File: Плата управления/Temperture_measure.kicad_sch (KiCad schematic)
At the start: 3 parts

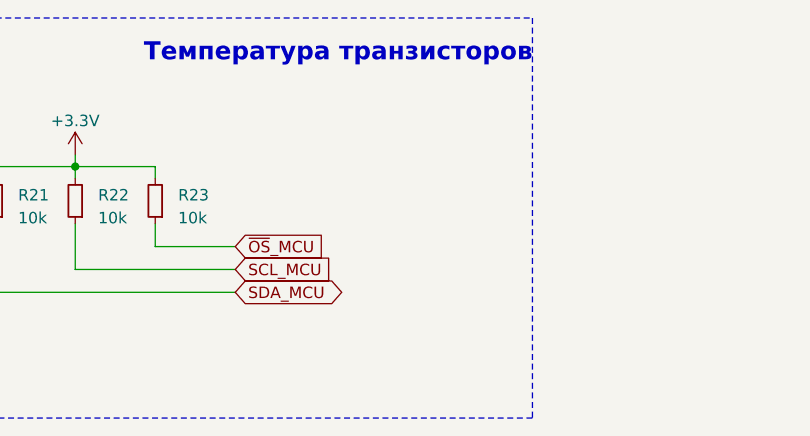
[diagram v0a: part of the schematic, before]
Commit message: Редактировал схему
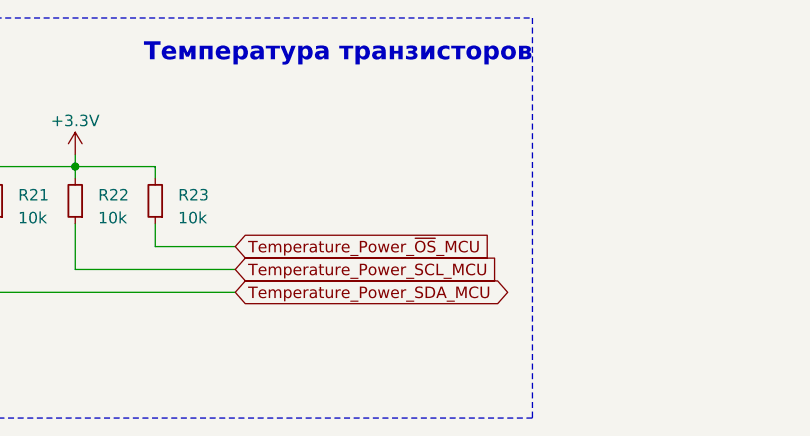
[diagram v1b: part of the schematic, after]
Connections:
- net SCL_MCU renamed Temperature_Power_SCL_MCU
- net SDA_MCU renamed Temperature_Power_SDA_MCU
- net ~{OS}_MCU renamed Temperature_Power_~{OS}_MCU
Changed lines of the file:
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@@
     (effects (font (size 2 2) bold) (justify left bottom))
   )
-  (global_label "SDA_MCU" (shape bidirectional) (at 74.93 45.72 0) (fields_autoplaced)
+  (global_label "Temperature_Power_SDA_MCU" (shape bidirectional) (at 74.93 45.72 0) (fields_autoplaced)
     (effects (font (size 1.27 1.27)) (justify left))
-    (property "Intersheetrefs" "${INTERSHEET_REFS}" (at 87.5347 45.72 0)
+    (property "Intersheetrefs" "${INTERSHEET_REFS}" (at 106.8454 45.72 0)
       (effects (font (size 1.27 1.27)) (justify left) hide)
     )
   )
-  (global_label "SCL_MCU" (shape input) (at 74.93 43.18 0) (fields_autoplaced)
+  (global_label "Temperature_Power_SCL_MCU" (shape input) (at 74.93 43.18 0) (fields_autoplaced)
     (effects (font (size 1.27 1.27)) (justify left))
-    (property "Intersheetrefs" "${INTERSHEET_REFS}" (at 86.3629 43.18 0)
+    (property "Intersheetrefs" "${INTERSHEET_REFS}" (at 105.6736 43.18 0)
       (effects (font (size 1.27 1.27)) (justify left) hide)
     )
   )
-  (global_label "~{OS}_MCU" (shape input) (at 74.93 40.64 0) (fields_autoplaced)
+  (global_label "Temperature_Power_~{OS}_MCU" (shape input) (at 74.93 40.64 0) (fields_autoplaced)
     (effects (font (size 1.27 1.27)) (justify left))
-    (property "Intersheetrefs" "${INTERSHEET_REFS}" (at 85.3953 40.64 0)
+    (property "Intersheetrefs" "${INTERSHEET_REFS}" (at 104.706 40.64 0)
       (effects (font (size 1.27 1.27)) (justify left) hide)
     )

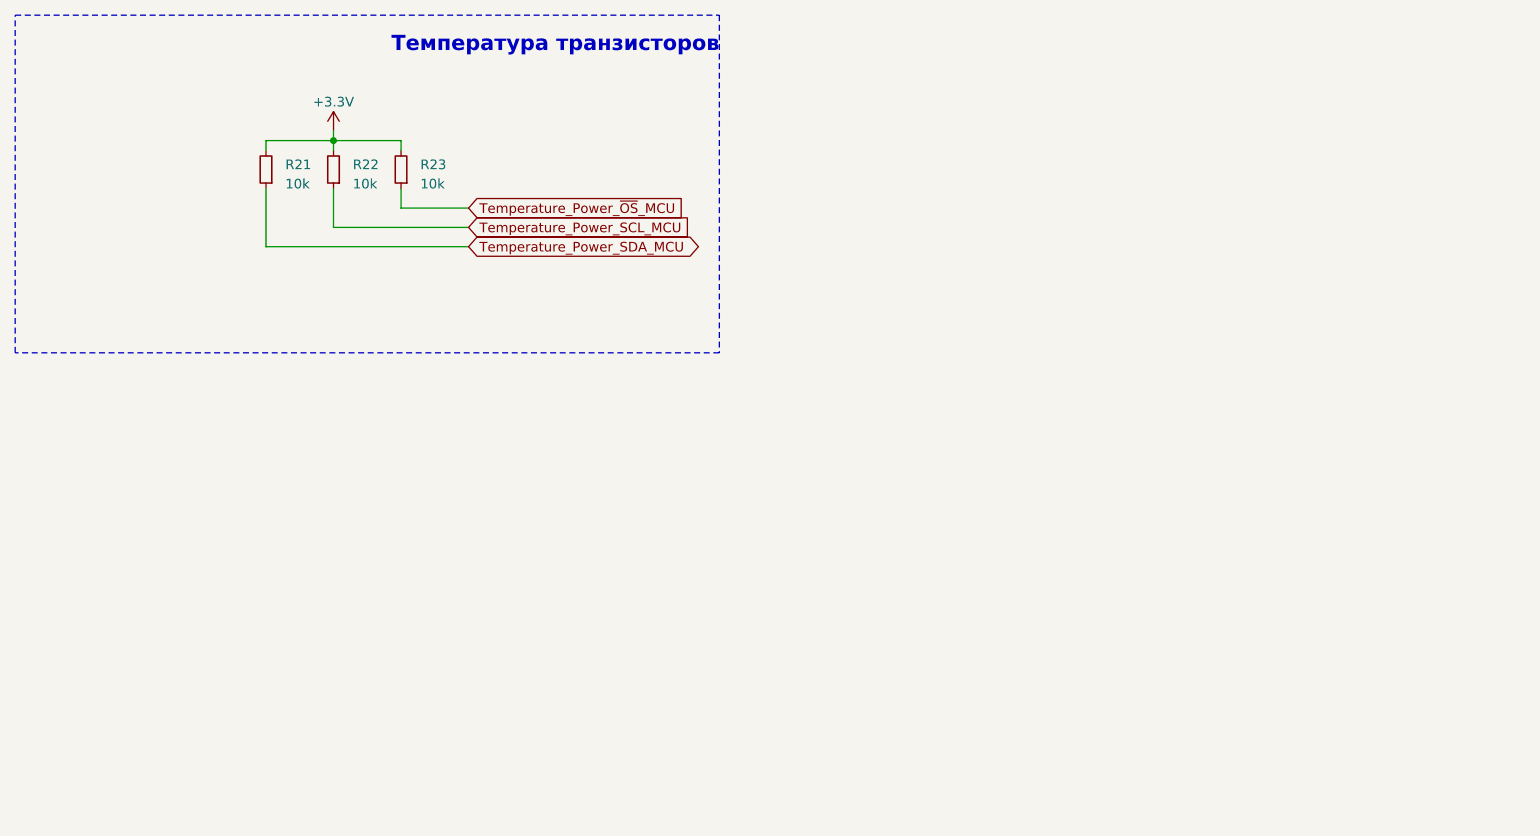
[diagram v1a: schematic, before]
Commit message: Добавил документы
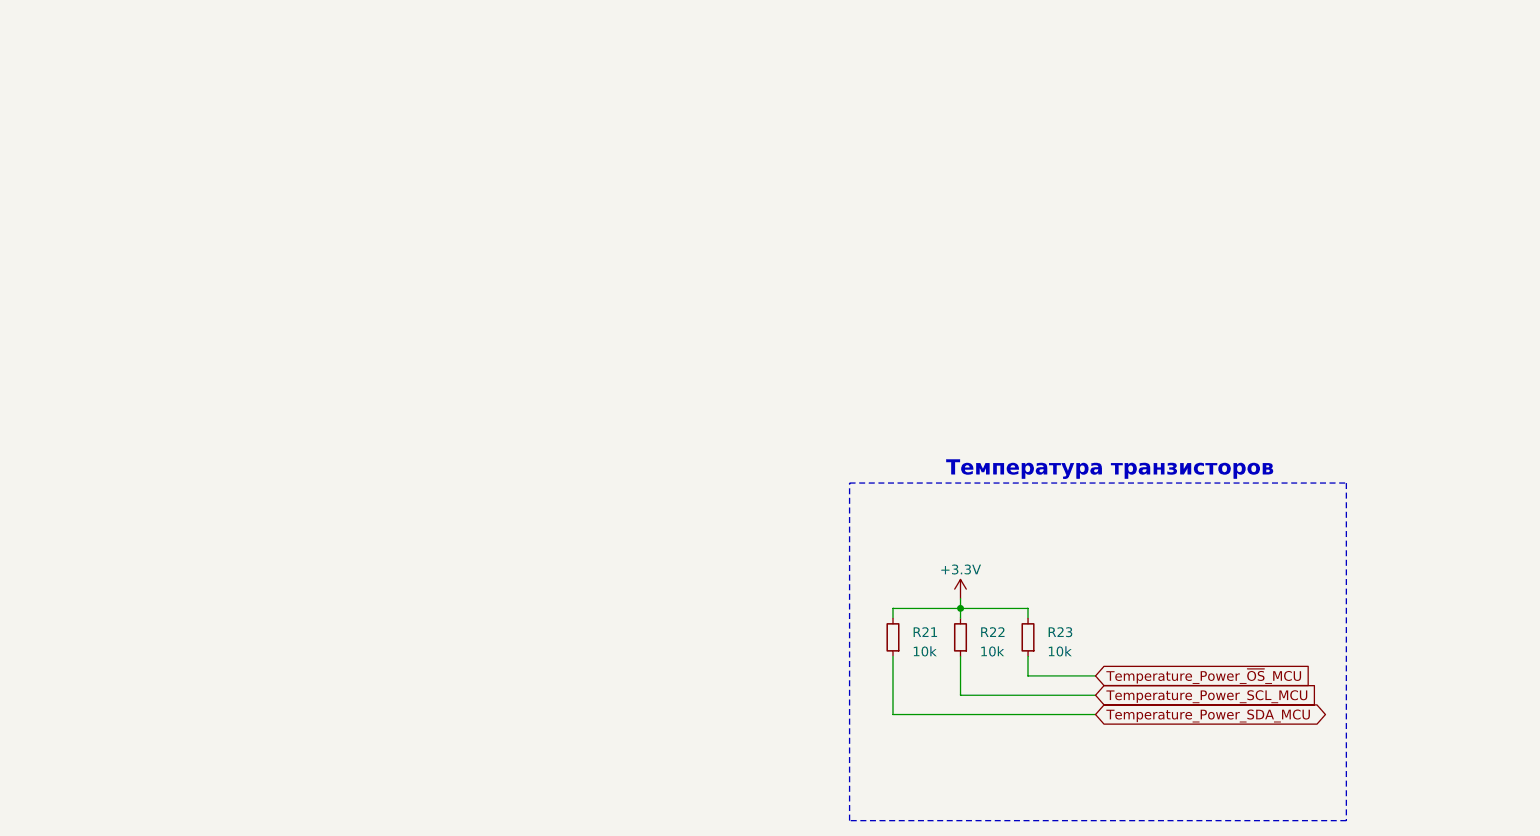
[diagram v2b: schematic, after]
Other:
- moved on the sheet: R21, R22, R23
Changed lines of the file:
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@@
 (kicad_sch (version 20230121) (generator eeschema)
   (paper "A4")
-  (junction (at 57.15 31.75) (diameter 0) (color 0 0 0 0)
+  (title_block
+    (comment 1 "МПСТ.76721.758764.02.Э3.М")
   )
-  (wire (pts (xy 74.93 45.72) (xy 48.26 45.72))
+  (junction (at 139.7 93.345) (diameter 0) (color 0 0 0 0)
+  )
+  (wire (pts (xy 157.48 107.315) (xy 130.81 107.315))
     (stroke (width 0) (type default))
   )
-  (wire (pts (xy 74.93 40.64) (xy 66.04 40.64))
+  (wire (pts (xy 157.48 102.235) (xy 148.59 102.235))
     (stroke (width 0) (type default))
   )
-  (wire (pts (xy 57.15 31.75) (xy 57.15 33.02))
+  (wire (pts (xy 139.7 93.345) (xy 139.7 94.615))
     (stroke (width 0) (type default))
   )
-  (wire (pts (xy 57.15 30.48) (xy 57.15 31.75))
+  (wire (pts (xy 139.7 92.075) (xy 139.7 93.345))
     (stroke (width 0) (type default))
   )
-  (wire (pts (xy 57.15 43.18) (xy 57.15 38.1))
+  (wire (pts (xy 139.7 104.775) (xy 139.7 99.695))
     (stroke (width 0) (type default))
   )
-  (wire (pts (xy 66.04 33.02) (xy 66.04 31.75))
+  (wire (pts (xy 148.59 94.615) (xy 148.59 93.345))
     (stroke (width 0) (type default))
   )
-  (wire (pts (xy 66.04 40.64) (xy 66.04 38.1))
+  (wire (pts (xy 148.59 102.235) (xy 148.59 99.695))
     (stroke (width 0) (type default))
   )
-  (wire (pts (xy 48.26 31.75) (xy 57.15 31.75))
+  (wire (pts (xy 130.81 93.345) (xy 139.7 93.345))
     (stroke (width 0) (type default))
   )
-  (wire (pts (xy 57.15 31.75) (xy 66.04 31.75))
+  (wire (pts (xy 139.7 93.345) (xy 148.59 93.345))
     (stroke (width 0) (type default))
   )
-  (wire (pts (xy 48.26 33.02) (xy 48.26 31.75))
+  (wire (pts (xy 130.81 94.615) (xy 130.81 93.345))
     (stroke (width 0) (type default))
   )
-  (wire (pts (xy 48.26 45.72) (xy 48.26 38.1))
+  (wire (pts (xy 130.81 107.315) (xy 130.81 99.695))
     (stroke (width 0) (type default))
   )
-  (wire (pts (xy 74.93 43.18) (xy 57.15 43.18))
+  (wire (pts (xy 157.48 104.775) (xy 139.7 104.775))
     (stroke (width 0) (type default))
   )
-  (rectangle (start 15.24 15.24) (end 107.95 59.69)
-    (stroke (width 0) (type dot))
+  (rectangle (start 125.095 76.835) (end 190.5 121.285)
+    (stroke (width 0) (type dash))
     (fill (type none))
   )
-  (text "Температура транзисторов" (at 64.77 20.32 0)
+  (text "Температура транзисторов" (at 137.795 76.2 0)
     (effects (font (size 2 2) bold) (justify left bottom))
   )
-  (global_label "Temperature_Power_SDA_MCU" (shape bidirectional) (at 74.93 45.72 0) (fields_autoplaced)
+  (global_label "Temperature_Power_SDA_MCU" (shape bidirectional) (at 157.48 107.315 0) (fields_autoplaced)
     (effects (font (size 1.27 1.27)) (justify left))
-    (property "Intersheetrefs" "${INTERSHEET_REFS}" (at 106.8454 45.72 0)
+    (property "Intersheetrefs" "${INTERSHEET_REFS}" (at 189.3954 107.315 0)
       (effects (font (size 1.27 1.27)) (justify left) hide)
     )
   )
-  (global_label "Temperature_Power_SCL_MCU" (shape input) (at 74.93 43.18 0) (fields_autoplaced)
+  (global_label "Temperature_Power_SCL_MCU" (shape input) (at 157.48 104.775 0) (fields_autoplaced)
     (effects (font (size 1.27 1.27)) (justify left))
-    (property "Intersheetrefs" "${INTERSHEET_REFS}" (at 105.6736 43.18 0)
+    (property "Intersheetrefs" "${INTERSHEET_REFS}" (at 188.2236 104.775 0)
       (effects (font (size 1.27 1.27)) (justify left) hide)
     )
   )
-  (global_label "Temperature_Power_~{OS}_MCU" (shape input) (at 74.93 40.64 0) (fields_autoplaced)
+  (global_label "Temperature_Power_~{OS}_MCU" (shape input) (at 157.48 102.235 0) (fields_autoplaced)
     (effects (font (size 1.27 1.27)) (justify left))
-    (property "Intersheetrefs" "${INTERSHEET_REFS}" (at 104.706 40.64 0)
+    (property "Intersheetrefs" "${INTERSHEET_REFS}" (at 187.256 102.235 0)
       (effects (font (size 1.27 1.27)) (justify left) hide)
     )
   )
-  (symbol (lib_id "Device:R_Small") (at 66.04 35.56 180) (unit 1)
+  (symbol (lib_id "Device:R_Small") (at 148.59 97.155 180) (unit 1)
     (in_bom yes) (on_board yes) (dnp no) (fields_autoplaced)
-    (property "Reference" "R23" (at 68.58 34.925 0)
+    (property "Reference" "R23" (at 151.13 96.52 0)
       (effects (font (size 1.27 1.27)) (justify right))
     )
-    (property "Value" "10k" (at 68.58 37.465 0)
+    (property "Value" "10k" (at 151.13 99.06 0)
       (effects (font (size 1.27 1.27)) (justify right))
     )
-    (property "Footprint" "Resistor_SMD:R_0603_1608Metric_Pad0.98x0.95mm_HandSolder" (at 66.04 35.56 0)
+    (property "Footprint" "Resistor_SMD:R_0603_1608Metric_Pad0.98x0.95mm_HandSolder" (at 148.59 97.155 0)
       (effects (font (size 1.27 1.27)) hide)
     )
-    (property "Datasheet" "~" (at 66.04 35.56 0)
+    (property "Datasheet" "~" (at 148.59 97.155 0)
       (effects (font (size 1.27 1.27)) hide)
     )
@@
     )
   )
-  (symbol (lib_id "power:+3.3V") (at 57.15 30.48 0) (unit 1)
+  (symbol (lib_id "power:+3.3V") (at 139.7 92.075 0) (unit 1)
     (in_bom yes) (on_board yes) (dnp no) (fields_autoplaced)
-    (property "Reference" "#PWR029" (at 57.15 34.29 0)
+    (property "Reference" "#PWR029" (at 139.7 95.885 0)
       (effects (font (size 1.27 1.27)) hide)
     )
-    (property "Value" "+3.3V" (at 57.15 26.67 0)
+    (property "Value" "+3.3V" (at 139.7 88.265 0)
       (effects (font (size 1.27 1.27)))
     )
-    (property "Footprint" "" (at 57.15 30.48 0)
+    (property "Footprint" "" (at 139.7 92.075 0)
       (effects (font (size 1.27 1.27)) hide)
     )
-    (property "Datasheet" "" (at 57.15 30.48 0)
+    (property "Datasheet" "" (at 139.7 92.075 0)
       (effects (font (size 1.27 1.27)) hide)
     )
@@
     )
   )
-  (symbol (lib_id "Device:R_Small") (at 48.26 35.56 180) (unit 1)
+  (symbol (lib_id "Device:R_Small") (at 130.81 97.155 180) (unit 1)
     (in_bom yes) (on_board yes) (dnp no) (fields_autoplaced)
-    (property "Reference" "R21" (at 50.8 34.925 0)
+    (property "Reference" "R21" (at 133.35 96.52 0)
       (effects (font (size 1.27 1.27)) (justify right))
     )
-    (property "Value" "10k" (at 50.8 37.465 0)
+    (property "Value" "10k" (at 133.35 99.06 0)
       (effects (font (size 1.27 1.27)) (justify right))
     )
-    (property "Footprint" "Resistor_SMD:R_0603_1608Metric_Pad0.98x0.95mm_HandSolder" (at 48.26 35.56 0)
+    (property "Footprint" "Resistor_SMD:R_0603_1608Metric_Pad0.98x0.95mm_HandSolder" (at 130.81 97.155 0)
       (effects (font (size 1.27 1.27)) hide)
     )
-    (property "Datasheet" "~" (at 48.26 35.56 0)
+    (property "Datasheet" "~" (at 130.81 97.155 0)
       (effects (font (size 1.27 1.27)) hide)
     )
@@
     )
   )
-  (symbol (lib_id "Device:R_Small") (at 57.15 35.56 180) (unit 1)
+  (symbol (lib_id "Device:R_Small") (at 139.7 97.155 180) (unit 1)
     (in_bom yes) (on_board yes) (dnp no) (fields_autoplaced)
-    (property "Reference" "R22" (at 59.69 34.925 0)
+    (property "Reference" "R22" (at 142.24 96.52 0)
       (effects (font (size 1.27 1.27)) (justify right))
     )
-    (property "Value" "10k" (at 59.69 37.465 0)
+    (property "Value" "10k" (at 142.24 99.06 0)
       (effects (font (size 1.27 1.27)) (justify right))
     )
-    (property "Footprint" "Resistor_SMD:R_0603_1608Metric_Pad0.98x0.95mm_HandSolder" (at 57.15 35.56 0)
+    (property "Footprint" "Resistor_SMD:R_0603_1608Metric_Pad0.98x0.95mm_HandSolder" (at 139.7 97.155 0)
       (effects (font (size 1.27 1.27)) hide)
     )
-    (property "Datasheet" "~" (at 57.15 35.56 0)
+    (property "Datasheet" "~" (at 139.7 97.155 0)
       (effects (font (size 1.27 1.27)) hide)
     )
